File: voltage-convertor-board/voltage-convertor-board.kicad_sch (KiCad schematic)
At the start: 78 parts, among them IC1 MCP2562, J1 Conn_01x04, J10 Conn_01x02, J11 Conn_01x02, J2 Conn_01x03, J3 Conn_01x03, J4 Conn_01x04, J5 Conn_01x04, J6 Conn_01x04_Pin, J7 Conn_01x04, J8 Conn_01x03, J9 Conn_01x03, Q1 BSS138, Q2 BSS138, Q3 BSS138, Q4 BSS138, SW1 SW_Push, U1 TPS54560BDDA, U2 NJM12888F33, U5 STM32G431K8Tx, U6 NJM7805SDL1

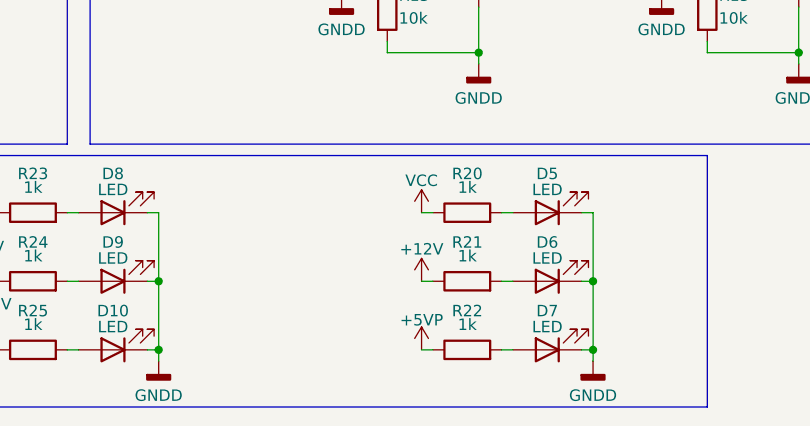
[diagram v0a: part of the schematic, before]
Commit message: 完成
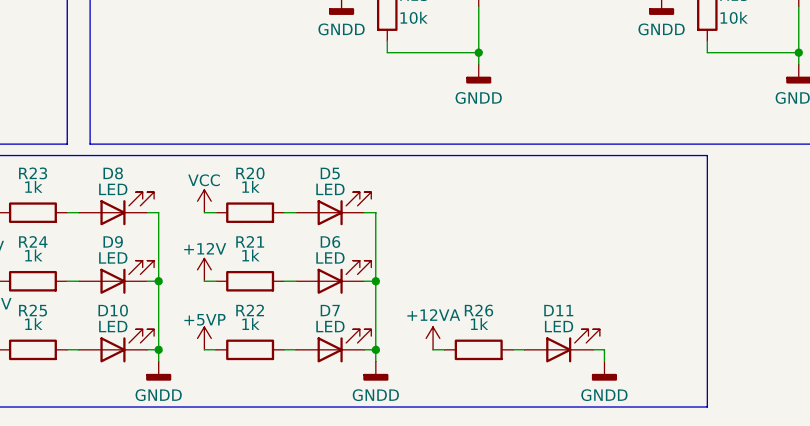
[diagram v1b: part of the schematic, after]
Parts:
- added D11: LED, LED_SMD:LED_0603_1608Metric_Pad1.05x0.95mm_HandSolder, symbol Device:LED
- added R26: 1k, Resistor_SMD:R_0603_1608Metric_Pad0.98x0.95mm_HandSolder, symbol Device:R
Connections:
- net +12VA: now also R26.1
- net GNDD: now also D11.1 (K)
- new net: D11.2 (A), R26.2
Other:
- moved on the sheet: D5, D6, D7, R20, R21, R22
